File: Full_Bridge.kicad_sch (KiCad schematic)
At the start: 8 parts, among them U19 DRV8838DSGT

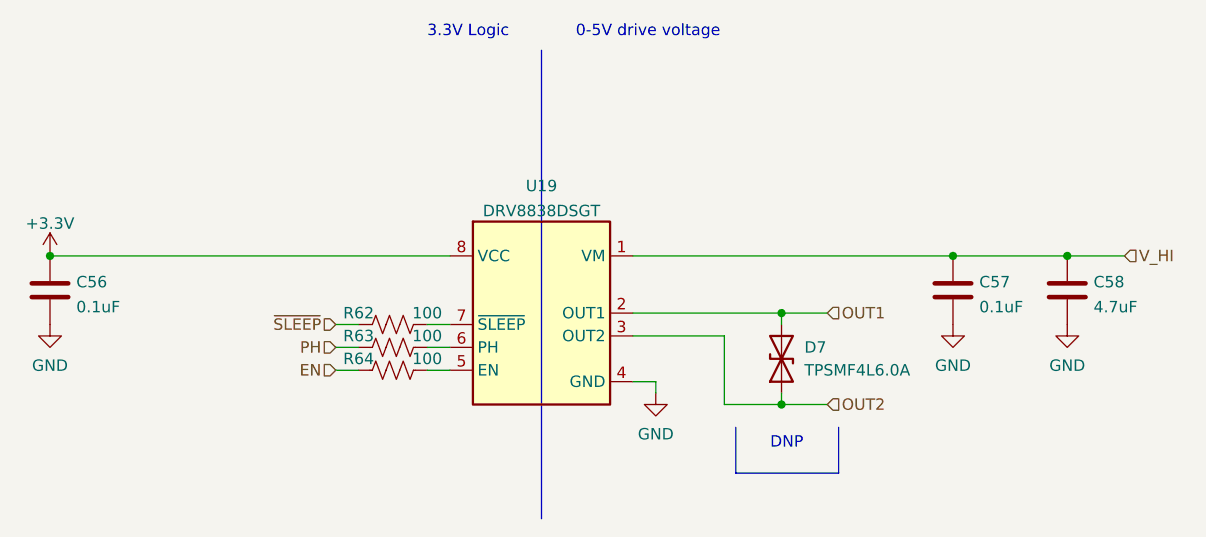
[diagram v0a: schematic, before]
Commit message: working on EM
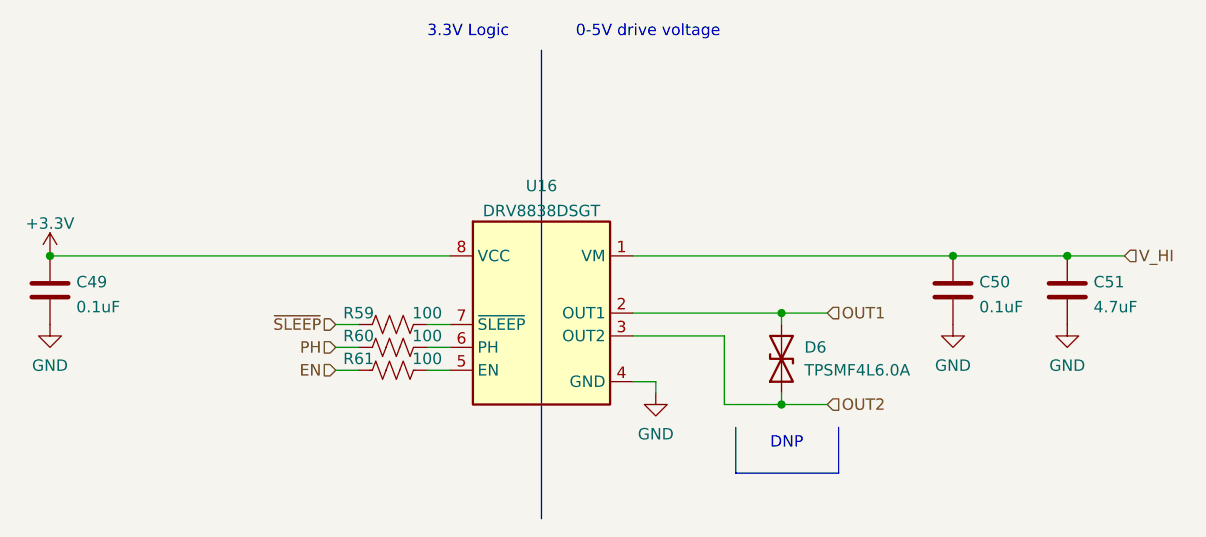
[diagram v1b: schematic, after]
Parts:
- renumbered C56 to C49, C57 to C50, C58 to C51, D7 to D6, R62 to R59, R63 to R60, R64 to R61, U19 to U16
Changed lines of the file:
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@@
   (symbol (lib_id "power:GND") (at 80.01 88.9 0)
     (in_bom yes) (on_board yes) (fields_autoplaced)
-    (property "Reference" "#PWR053" (id 0) (at 80.01 95.25 0)
+    (property "Reference" "#PWR044" (id 0) (at 80.01 95.25 0)
       (effects (font (size 1.27 1.27)) hide)
     )
@@
   (symbol (lib_id "Device:D_TVS") (at 161.29 92.71 90)
     (in_bom yes) (on_board yes) (fields_autoplaced)
-    (property "Reference" "D7" (id 0) (at 163.83 91.4399 90)
+    (property "Reference" "D6" (id 0) (at 163.83 91.4399 90)
       (effects (font (size 1.27 1.27)) (justify right))
     )
@@
   (symbol (lib_id "Device:C") (at 80.01 85.09 0)
     (in_bom yes) (on_board yes) (fields_autoplaced)
-    (property "Reference" "C56" (id 0) (at 82.931 84.1815 0)
+    (property "Reference" "C49" (id 0) (at 82.931 84.1815 0)
       (effects (font (size 1.27 1.27)) (justify left))
     )
@@
   (symbol (lib_id "Device:R_US") (at 118.11 91.44 90)
     (in_bom yes) (on_board yes)
-    (property "Reference" "R63" (id 0) (at 114.3 90.17 90))
+    (property "Reference" "R60" (id 0) (at 114.3 90.17 90))
     (property "Value" "100" (id 1) (at 121.92 90.17 90))
     (property "Footprint" "Resistor_SMD:R_0603_1608Metric" (id 2) (at 118.364 90.424 90)
@@
   (symbol (lib_id "power:GND") (at 193.04 88.9 0)
     (in_bom yes) (on_board yes) (fields_autoplaced)
-    (property "Reference" "#PWR056" (id 0) (at 193.04 95.25 0)
+    (property "Reference" "#PWR047" (id 0) (at 193.04 95.25 0)
       (effects (font (size 1.27 1.27)) hide)
     )
@@
   (symbol (lib_id "power:GND") (at 147.32 96.52 0)
     (in_bom yes) (on_board yes) (fields_autoplaced)
-    (property "Reference" "#PWR054" (id 0) (at 147.32 102.87 0)
+    (property "Reference" "#PWR045" (id 0) (at 147.32 102.87 0)
       (effects (font (size 1.27 1.27)) hide)
     )
@@
   (symbol (lib_id "power:GND") (at 180.34 88.9 0)
     (in_bom yes) (on_board yes) (fields_autoplaced)
-    (property "Reference" "#PWR055" (id 0) (at 180.34 95.25 0)
+    (property "Reference" "#PWR046" (id 0) (at 180.34 95.25 0)
       (effects (font (size 1.27 1.27)) hide)
     )
@@
   (symbol (lib_id "Device:R_US") (at 118.11 93.98 90)
     (in_bom yes) (on_board yes)
-    (property "Reference" "R64" (id 0) (at 114.3 92.71 90))
+    (property "Reference" "R61" (id 0) (at 114.3 92.71 90))
     (property "Value" "100" (id 1) (at 121.92 92.71 90))
     (property "Footprint" "Resistor_SMD:R_0603_1608Metric" (id 2) (at 118.364 92.964 90)
@@
   (symbol (lib_id "magnetotorquer-test-board:DRV8838DSGT") (at 134.62 87.63 0)
     (in_bom yes) (on_board yes) (fields_autoplaced)
-    (property "Reference" "U19" (id 0) (at 134.62 73.5035 0))
+    (property "Reference" "U16" (id 0) (at 134.62 73.5035 0))
     (property "Value" "DRV8838DSGT" (id 1) (at 134.62 76.2786 0))
     (property "Footprint" "Package_SON:WSON-8-1EP_2x2mm_P0.5mm_EP0.9x1.6mm" (id 2) (at 134.62 109.22 0)
@@
   (symbol (lib_id "Device:R_US") (at 118.11 88.9 90)
     (in_bom yes) (on_board yes)
-    (property "Reference" "R62" (id 0) (at 114.3 87.63 90))
+    (property "Reference" "R59" (id 0) (at 114.3 87.63 90))
     (property "Value" "100" (id 1) (at 121.92 87.63 90))
     (property "Footprint" "Resistor_SMD:R_0603_1608Metric" (id 2) (at 118.364 87.884 90)
@@
   (symbol (lib_id "power:+3.3V") (at 80.01 81.28 0)
     (in_bom yes) (on_board yes) (fields_autoplaced)
-    (property "Reference" "#PWR052" (id 0) (at 80.01 85.09 0)
+    (property "Reference" "#PWR043" (id 0) (at 80.01 85.09 0)
       (effects (font (size 1.27 1.27)) hide)
     )
@@
   (symbol (lib_id "Device:C") (at 180.34 85.09 0)
     (in_bom yes) (on_board yes) (fields_autoplaced)
-    (property "Reference" "C57" (id 0) (at 183.261 84.1815 0)
+    (property "Reference" "C50" (id 0) (at 183.261 84.1815 0)
       (effects (font (size 1.27 1.27)) (justify left))
     )
@@
   (symbol (lib_id "Device:C") (at 193.04 85.09 0)
     (in_bom yes) (on_board yes) (fields_autoplaced)
-    (property "Reference" "C58" (id 0) (at 195.961 84.1815 0)
+    (property "Reference" "C51" (id 0) (at 195.961 84.1815 0)
       (effects (font (size 1.27 1.27)) (justify left))
     )
